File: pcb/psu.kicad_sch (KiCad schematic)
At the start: 8 parts

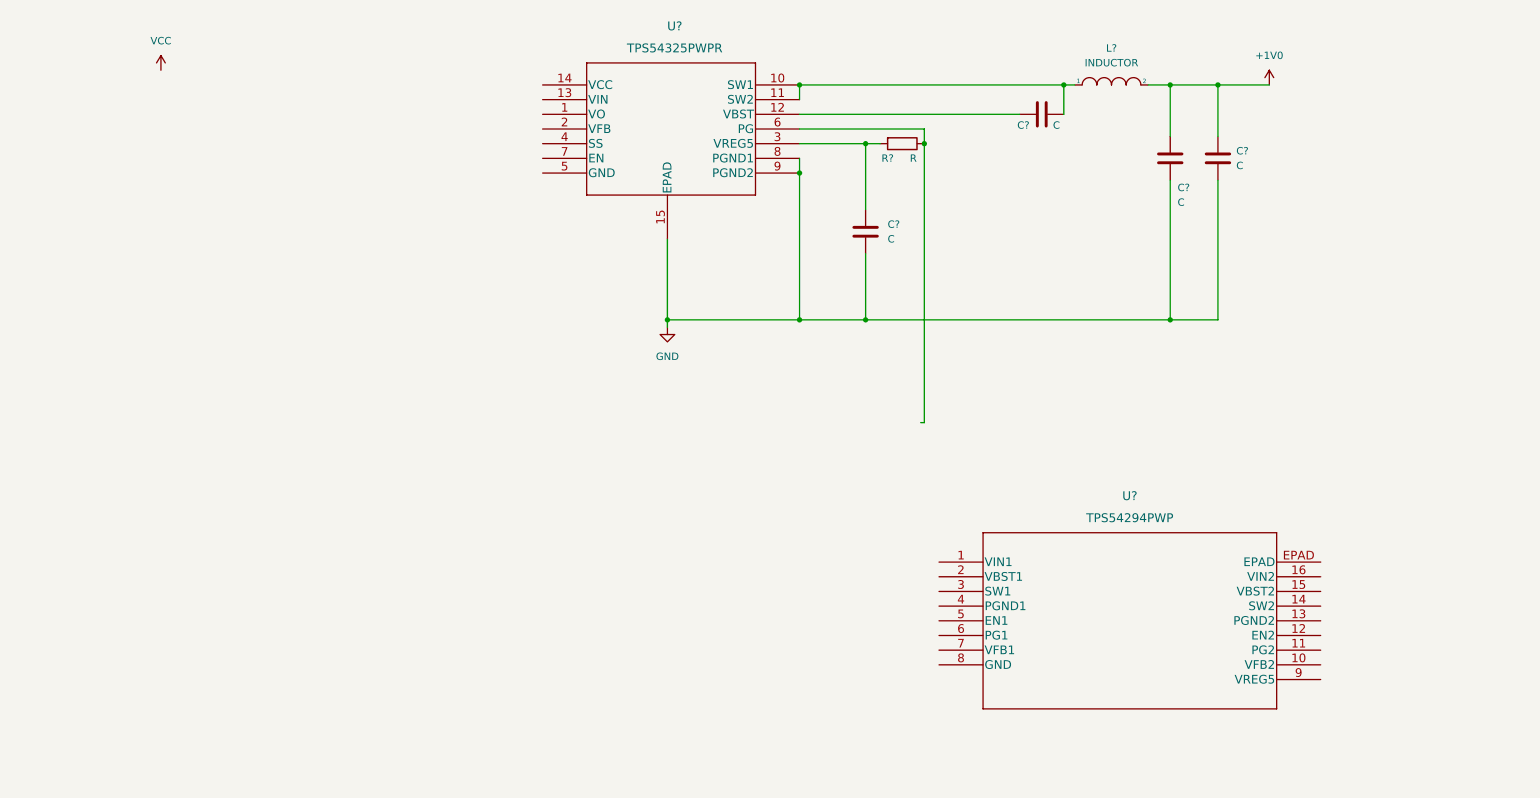
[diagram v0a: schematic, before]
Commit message: more work on psu
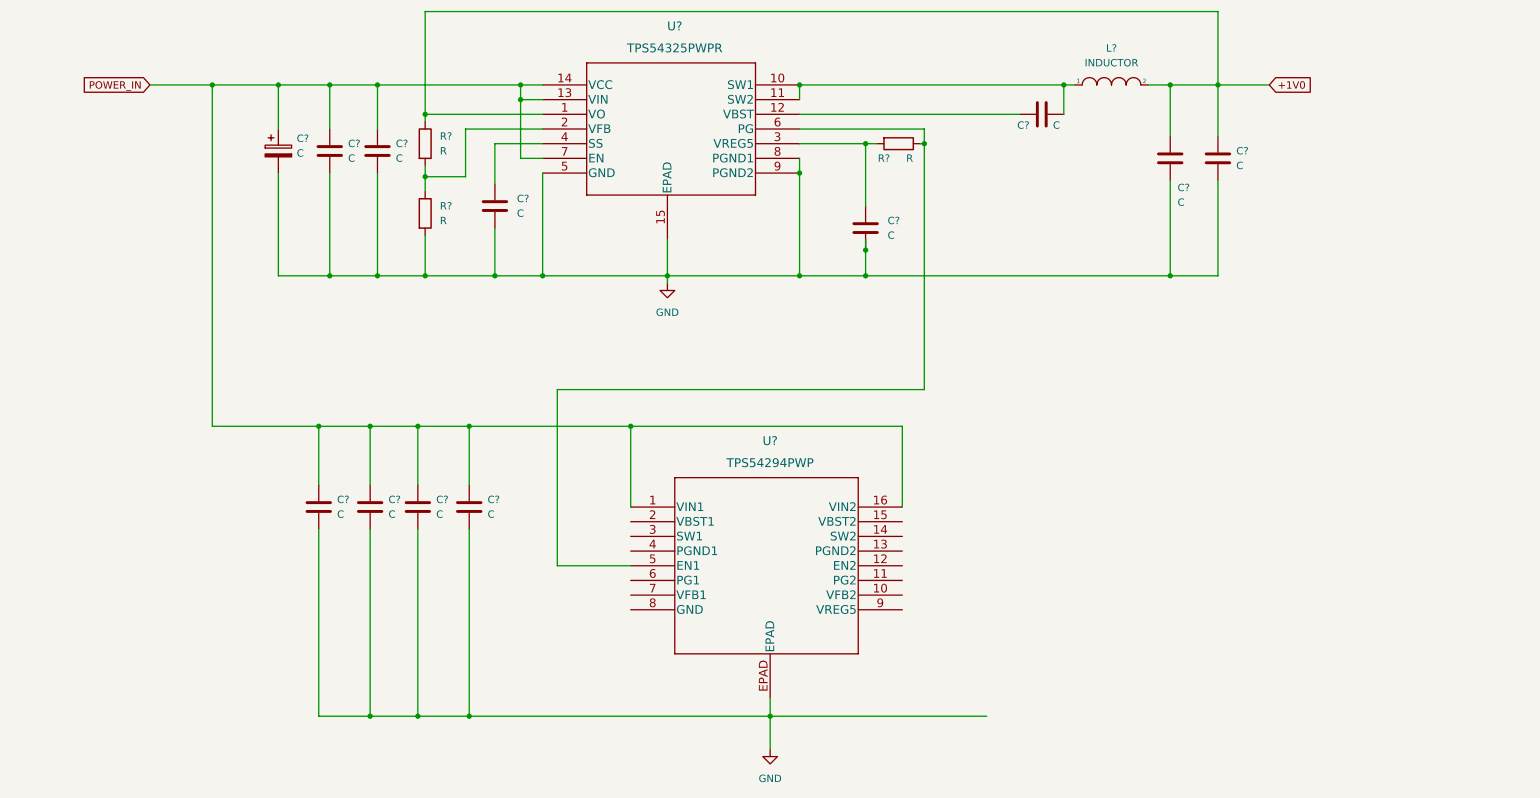
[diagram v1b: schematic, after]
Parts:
- added C? (x7): C, symbol Device:C
- added C?: C, symbol Device:C_Polarized
- added R? (x2): R, symbol Device:R
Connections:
- net +1V0: now also U?.1 (VO), R?.1
- net GND: now also U?.5 (GND), U?.EPAD, C?.2, C?.2, C?.2, C?.2, C?.2, C?.2, C?.2, C?.2, R?.2
- net at R?.1, U?.6 (PG): now also U?.5 (EN1)
- net POWER_IN: now reaches U?.1 (VIN1)
- net POWER_IN: now also U?.13 (VIN), U?.14 (VCC), U?.16 (VIN2), U?.7 (EN), C?.1, C?.1, C?.1, C?.1, C?.1, C?.1, C?.1
- net at U?.2 (VFB): now also R?.1, R?.2
- net at U?.4 (SS): now also C?.1
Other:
- moved on the sheet: C?, R?, U?

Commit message: finish wiring
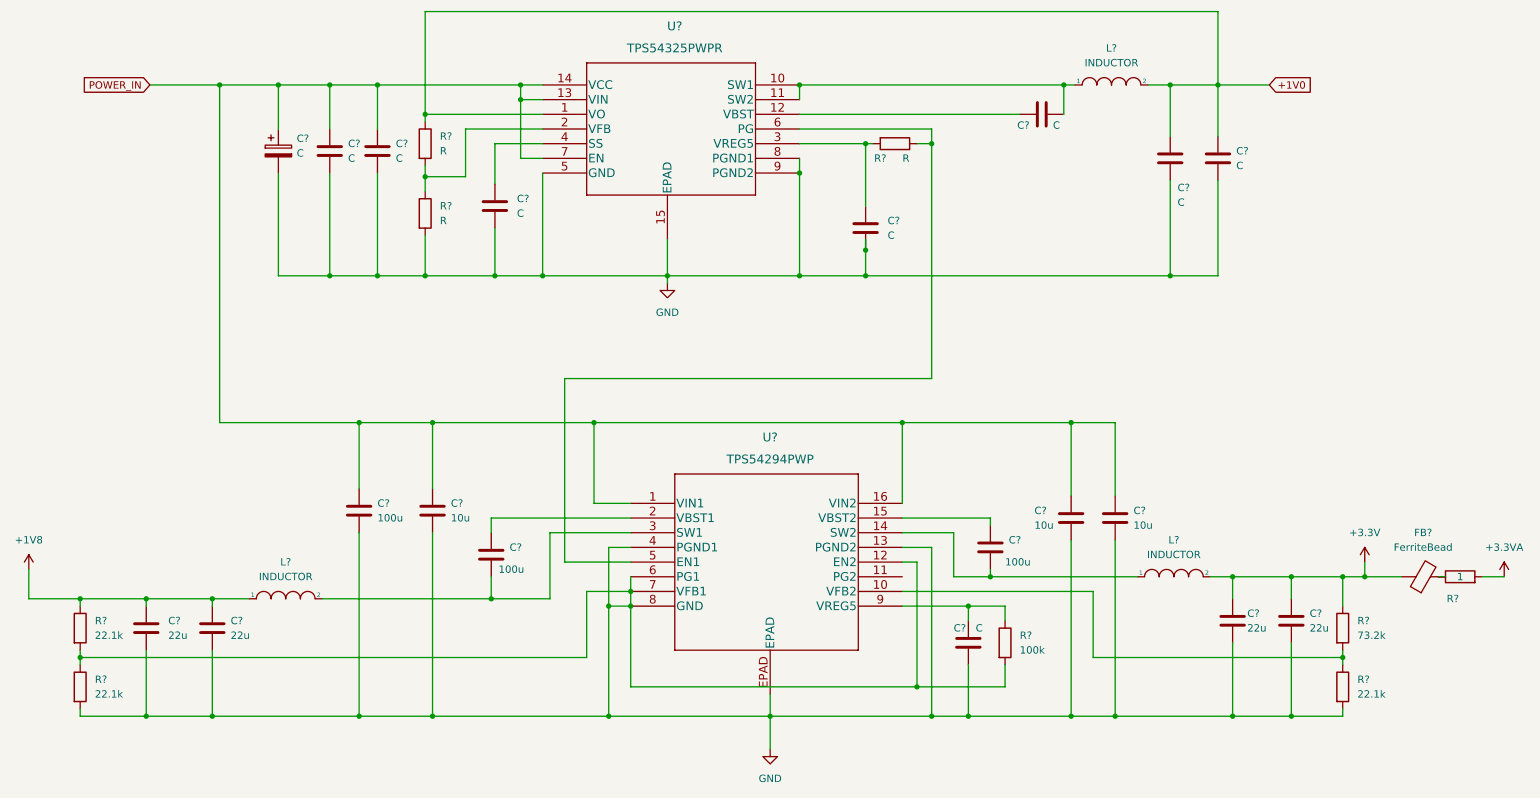
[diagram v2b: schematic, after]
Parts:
- added C? (x4): 22u, symbol Device:C
- added C? (x2): 100u, symbol Device:C
- added C?: C, symbol Device:C
- added FB?: FerriteBead, symbol Device:FerriteBead
- added L? (x2): INDUCTOR, symbol pspice:INDUCTOR
- added R? (x3): 22.1k, symbol Device:R
- added R?: 100k, symbol Device:R
- added R?: 73.2k, symbol Device:R
- added R?: 1, symbol Device:R
- C? (x3): value C -> 10u
- C?: value C -> 100u
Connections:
- net GND: now also U?.12 (EN2), U?.13 (PGND2), U?.4 (PGND1), U?.6 (PG1), U?.7 (VFB1), U?.8 (GND), C?.2, C?.2, C?.2, C?.2, C?.2, R?.1, R?.2, R?.2, R?.2, R?.2
- net at U?.10 (VFB2): now also R?.1, R?.2
- net at U?.14 (SW2): now also C?.2, L?.1
- net at U?.15 (VBST2): now also C?.1
- net at U?.2 (VBST1): now also C?.1
- net at U?.3 (SW1): now also C?.2, L?.2
- net at U?.9 (VREG5): now also C?.1, R?.1
- new net: FB?.2, R?.1
- new net +1V8: C?.1, C?.1, L?.1, R?.1
- new net +3.3V: C?.1, C?.1, FB?.1, L?.2, R?.1
- new net +3.3VA: R?.2
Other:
- moved on the sheet: C?, R?, U?
